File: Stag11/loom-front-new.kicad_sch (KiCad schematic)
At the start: 8 parts

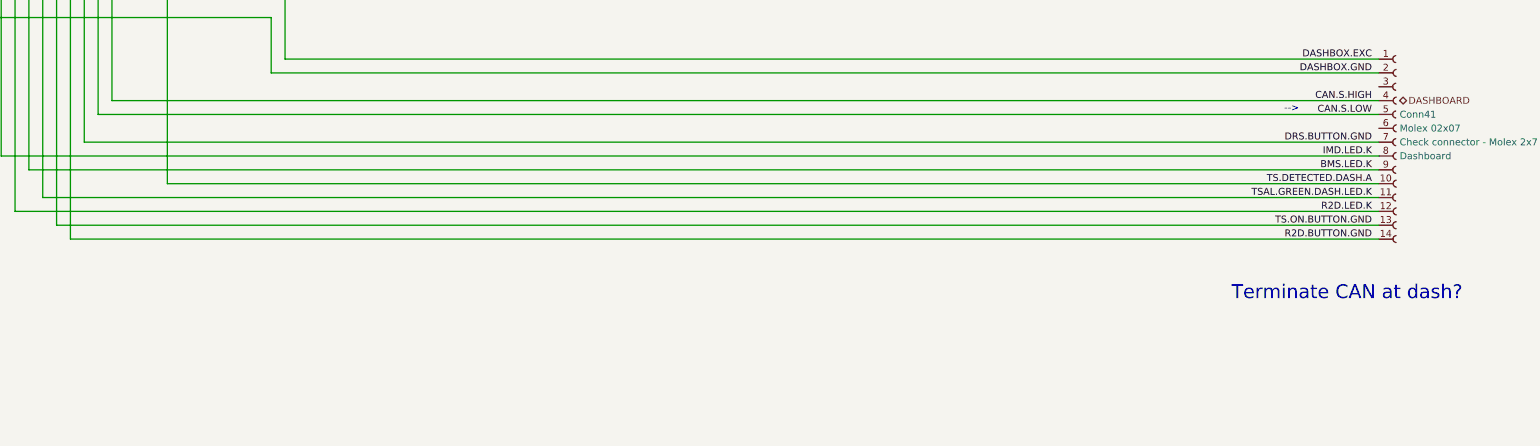
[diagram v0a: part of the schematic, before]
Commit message: I forgot what I did but changed CAN layout
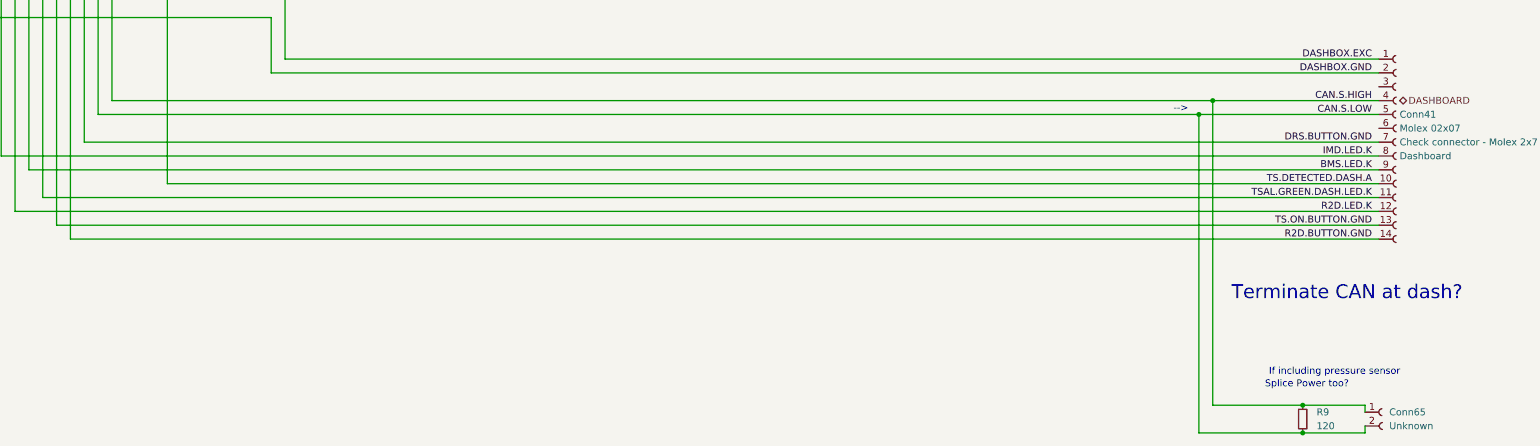
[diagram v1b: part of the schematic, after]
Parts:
- added Conn65: Deutsch_DTM_2S_Pin, symbol Connectors_SUFST:Deutsch_DTM_2S_Pin
- added R9: 120, symbol Device:R_Small
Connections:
- net CAN.S.HIGH: now also Conn65.1, R9.1
- net CAN.S.LOW: now also Conn65.2, R9.2
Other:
- note added: "If including pressure sensor"
- note added: "Splice Power too?"
